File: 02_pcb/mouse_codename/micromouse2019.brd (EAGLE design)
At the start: 45 x 50 mm, 80 parts

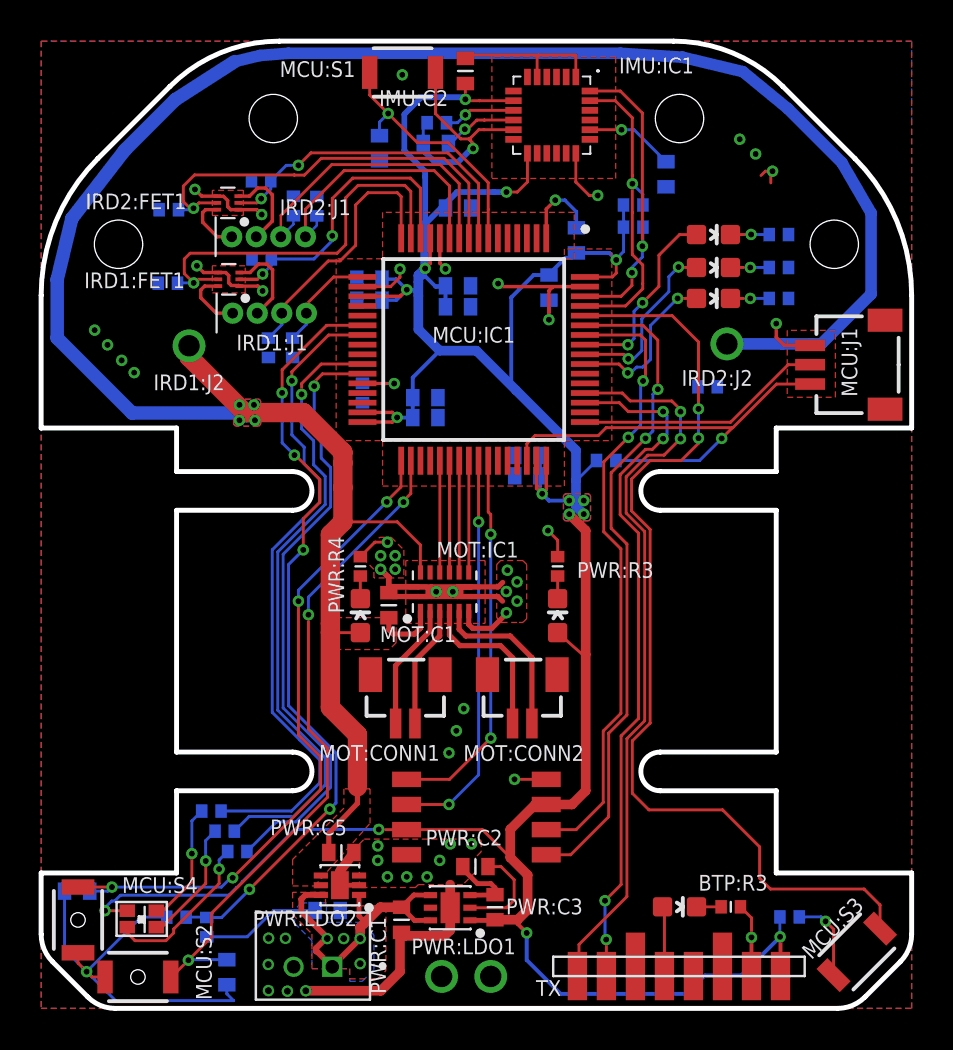
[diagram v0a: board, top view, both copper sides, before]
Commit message: minior fixes
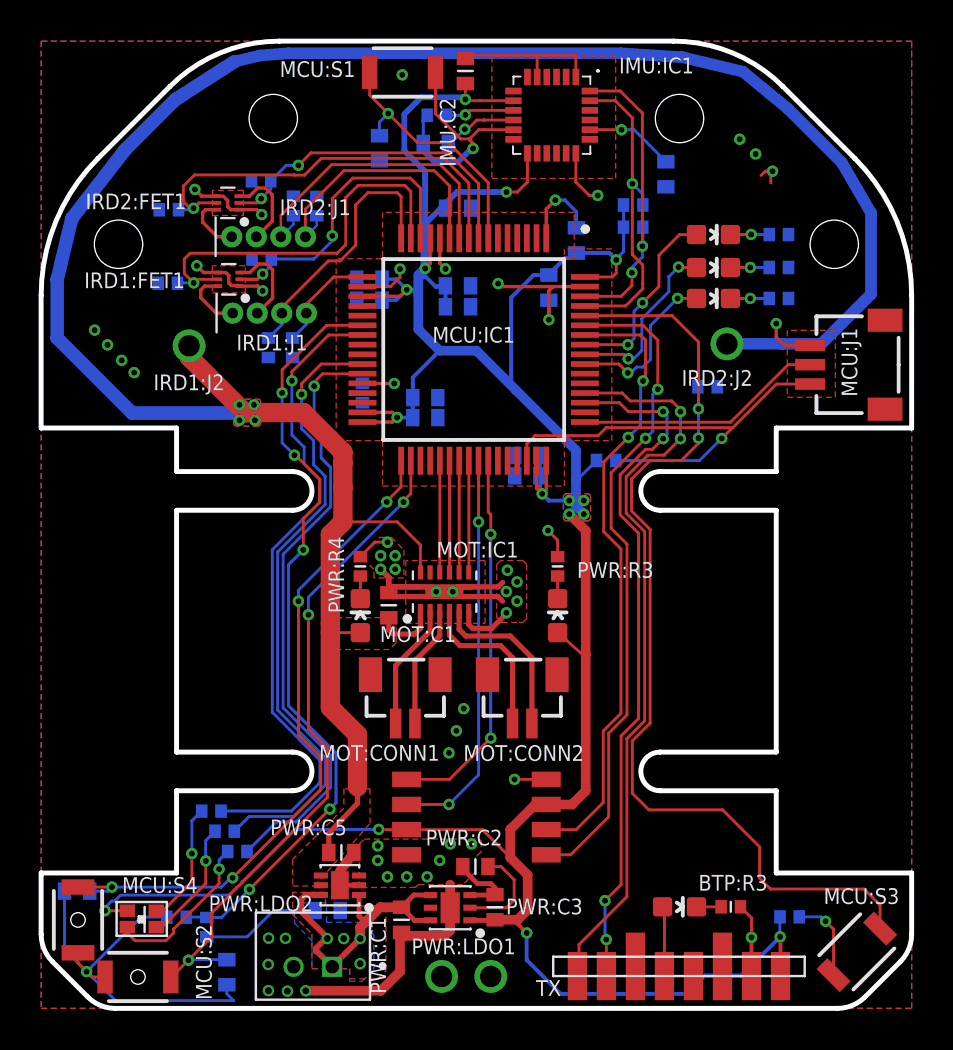
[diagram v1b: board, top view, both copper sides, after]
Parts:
- moved IMU:R1 0.38 mm to (20.5, 46.2)
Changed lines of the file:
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@@
 <layer number="132" name="bAdjust" color="7" fill="1" visible="no" active="yes"/>
 <layer number="144" name="Drill_legend" color="7" fill="1" visible="no" active="yes"/>
-<layer number="150" name="Notes" color="7" fill="1" visible="no" active="yes"/>
+<layer number="150" name="Notes" color="7" fill="1" visible="yes" active="yes"/>
 <layer number="151" name="HeatSink" color="7" fill="1" visible="no" active="yes"/>
 <layer number="152" name="_bDocu" color="7" fill="1" visible="no" active="yes"/>
@@
 <attribute name="MANUFACTURER_PART_NUMBER" value="B3U-1000P" x="42.164" y="2.921" size="1.778" layer="27" rot="R45" display="off"/>
 <attribute name="MOUSER_PART_NUMBER" value="653-B3U-1000P" x="42.164" y="2.921" size="1.778" layer="27" rot="R45" display="off"/>
-<attribute name="NAME" x="40.9124125" y="4.15563125" size="0.8128" layer="25" rot="R45" align="center"/>
+<attribute name="NAME" x="42.406009375" y="5.80396875" size="0.8128" layer="25" align="center"/>
 <attribute name="VALUE" x="43.240896875" y="1.01255" size="1.27" layer="27" rot="R45" align="center"/>
 </element>
@@
 </element>
 <element name="MCU:C11" library="0-micromouse2019" package="C0402" package3d_urn="urn:adsk.eagle:package:23626/2" value="100n" x="17.49" y="44.465" smashed="yes" rot="MR270">
-<attribute name="NAME" x="16.165" y="41.387" size="0.8128" layer="26" rot="MR90"/>
+<attribute name="NAME" x="15.911" y="40.752" size="0.8128" layer="26" rot="MR90"/>
 <attribute name="SPICEPREFIX" value="C" x="98.77" y="57.165" size="1.778" layer="28" rot="MR270" display="off"/>
 <attribute name="VALUE" x="19.014" y="46.243" size="0.8128" layer="28" rot="MR270"/>
@@
 <attribute name="VALUE" x="33.824" y="44.898" size="0.8128" layer="28" rot="MR270"/>
 </element>
-<element name="IMU:R1" library="0-micromouse2019" package="R0402" package3d_urn="urn:adsk.eagle:package:23547/3" value="47k" x="20.454" y="45.785" smashed="yes" rot="MR180">
-<attribute name="NAME" x="26.022" y="45.384" size="0.8128" layer="26" rot="MR0"/>
-<attribute name="SPICEPREFIX" value="R" x="20.454" y="45.785" size="1.778" layer="28" rot="MR180" display="off"/>
-<attribute name="VALUE" x="19.819" y="47.182" size="0.8128" layer="28" rot="MR180"/>
+<element name="IMU:R1" library="0-micromouse2019" package="R0402" package3d_urn="urn:adsk.eagle:package:23547/3" value="47k" x="20.454" y="46.166" smashed="yes" rot="MR180">
+<attribute name="NAME" x="26.022" y="45.765" size="0.8128" layer="26" rot="MR0"/>
+<attribute name="SPICEPREFIX" value="R" x="20.454" y="46.166" size="1.778" layer="28" rot="MR180" display="off"/>
+<attribute name="VALUE" x="19.819" y="47.563" size="0.8128" layer="28" rot="MR180"/>
 </element>
 <element name="IMU:C4" library="0-micromouse2019" package="C0402" package3d_urn="urn:adsk.eagle:package:23626/2" value="10n" x="21.553" y="41.372" smashed="yes" rot="MR180">
@@
 </element>
 <element name="IMU:C2" library="0-micromouse2019" package="C0402" package3d_urn="urn:adsk.eagle:package:23626/2" value="100n" x="21.93" y="48.458" smashed="yes" rot="R90">
-<attribute name="NAME" x="17.47" y="46.65" size="0.8128" layer="25"/>
+<attribute name="NAME" x="21.422" y="43.505" size="0.8128" layer="25" rot="R90"/>
 <attribute name="SPICEPREFIX" value="C" x="21.93" y="48.458" size="1.778" layer="27" rot="R90" display="off"/>
 <attribute name="VALUE" x="23.835" y="47.823" size="1.27" layer="27" rot="R90"/>
@@
 </element>
 <element name="PWR:LDO2" library="0-micromouse2019" package="SON50P200X200X80-7T92X145" package3d_urn="urn:adsk.eagle:package:9227372/1" value="PS_LDL112PU" x="15.445" y="6.367" smashed="yes" rot="R180">
-<attribute name="NAME" x="16.3365" y="5.0655" size="0.8128" layer="25" rot="R180"/>
+<attribute name="NAME" x="14.0505" y="5.8275" size="0.8128" layer="25" rot="R180"/>
 </element>
 <element name="PWR:LDO1" library="0-micromouse2019" package="SON65P200X200X80-7T100X160" package3d_urn="urn:adsk.eagle:package:9228423/1" value="PS_TPS735DRVT" x="21.144" y="5.203" smashed="yes" rot="R180">
@@
 </element>
 <element name="MCU:R4" library="0-micromouse2019" package="R0402" package3d_urn="urn:adsk.eagle:package:23547/3" value="270R" x="8.8" y="10.2" smashed="yes" rot="MR0">
-<attribute name="NAME" x="14.515" y="9.819" size="0.8128" layer="26" rot="MR0"/>
+<attribute name="NAME" x="14.261" y="9.819" size="0.8128" layer="26" rot="MR0"/>
 <attribute name="SPICEPREFIX" value="R" x="8.8" y="10.2" size="1.778" layer="28" rot="MR0" display="off"/>
 <attribute name="VALUE" x="9.435" y="8.803" size="0.8128" layer="28" rot="MR0"/>
@@
 </element>
 <element name="IRD1:R5" library="0-micromouse2019" package="R0402" package3d_urn="urn:adsk.eagle:package:23547/3" value="2R" x="11.75" y="34.15" smashed="yes" rot="MR90">
-<attribute name="NAME" x="11.623" y="28.943" size="0.8128" layer="26" rot="MR90"/>
+<attribute name="NAME" x="11.824" y="32.324" size="0.8128" layer="26" rot="MR0"/>
 <attribute name="SPICEPREFIX" value="R" x="11.75" y="34.15" size="1.778" layer="28" rot="MR90" display="off"/>
 <attribute name="VALUE" x="10.353" y="33.515" size="0.8128" layer="28" rot="MR90"/>
 </element>
 <element name="IRD1:R6" library="0-micromouse2019" package="R0402" package3d_urn="urn:adsk.eagle:package:23547/3" value="2R" x="13" y="34.15" smashed="yes" rot="MR90">
-<attribute name="NAME" x="12.492" y="28.943" size="0.8128" layer="26" rot="MR90"/>
+<attribute name="NAME" x="13.703" y="34.244" size="0.8128" layer="26" rot="MR180"/>
 <attribute name="SPICEPREFIX" value="R" x="13" y="34.15" size="1.778" layer="28" rot="MR90" display="off"/>
 <attribute name="VALUE" x="11.603" y="33.515" size="0.8128" layer="28" rot="MR90"/>
@@
 <wire x1="22.162" y1="46.422" x2="21.93" y2="46.19" width="0.1524" layer="1"/>
 <via x="21.93" y="46.19" extent="1-16" drill="0.3" diameter="0.6"/>
-<wire x1="21.93" y1="46.19" x2="21.525" y2="45.785" width="0.1524" layer="16"/>
-<wire x1="21.525" y1="45.785" x2="20.954" y2="45.785" width="0.1524" layer="16"/>
+<wire x1="21.93" y1="46.19" x2="21.906" y2="46.166" width="0.1524" layer="16"/>
+<wire x1="21.906" y1="46.166" x2="20.954" y2="46.166" width="0.1524" layer="16"/>
 <wire x1="24.415" y1="46.422" x2="22.162" y2="46.422" width="0.1524" layer="1"/>
 </signal>
@@
 <wire x1="25.64" y1="49.22" x2="25.64" y2="48.147" width="0.1524" layer="1"/>
 <wire x1="27.64" y1="49.28" x2="27.64" y2="48.147" width="0.1524" layer="1"/>
-<wire x1="19.753" y1="44.712" x2="19.753" y2="45.584" width="0.1524" layer="16"/>
-<wire x1="19.753" y1="45.584" x2="19.954" y2="45.785" width="0.1524" layer="16"/>
+<wire x1="19.753" y1="44.712" x2="19.753" y2="45.965" width="0.1524" layer="16"/>
+<wire x1="19.753" y1="45.965" x2="19.954" y2="46.166" width="0.1524" layer="16"/>
 <wire x1="19.753" y1="44.712" x2="19.753" y2="44.347" width="0.1524" layer="16"/>
 <wire x1="19.753" y1="44.347" x2="20.35" y2="43.75" width="0.3" layer="16"/>
